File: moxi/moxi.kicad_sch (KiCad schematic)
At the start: 7 parts, among them M3 Motor_Servo, M4 Motor_Servo, SW1 SW_SPST, U1 MAX98357A, U2 ProMicro_2

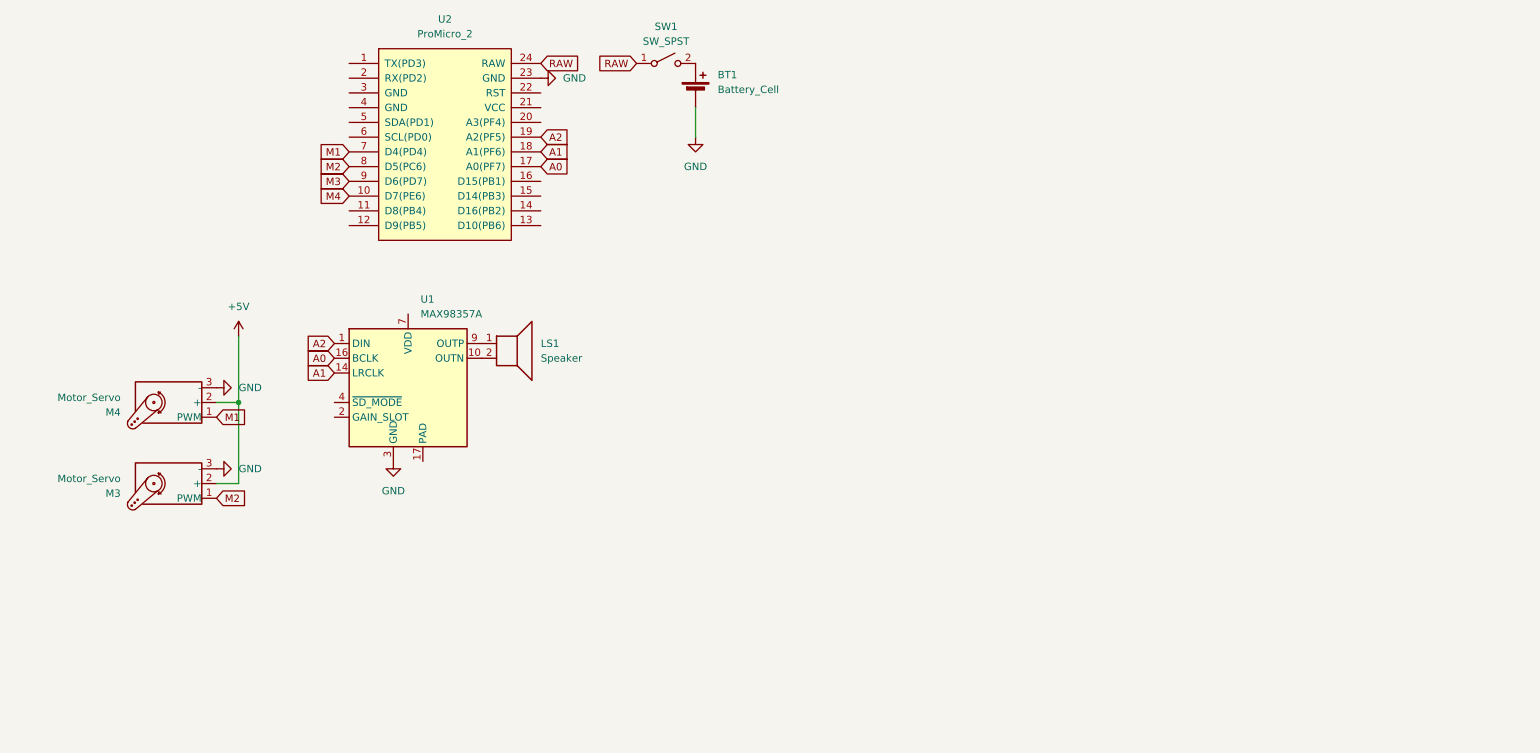
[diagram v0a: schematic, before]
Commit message: Update schematic
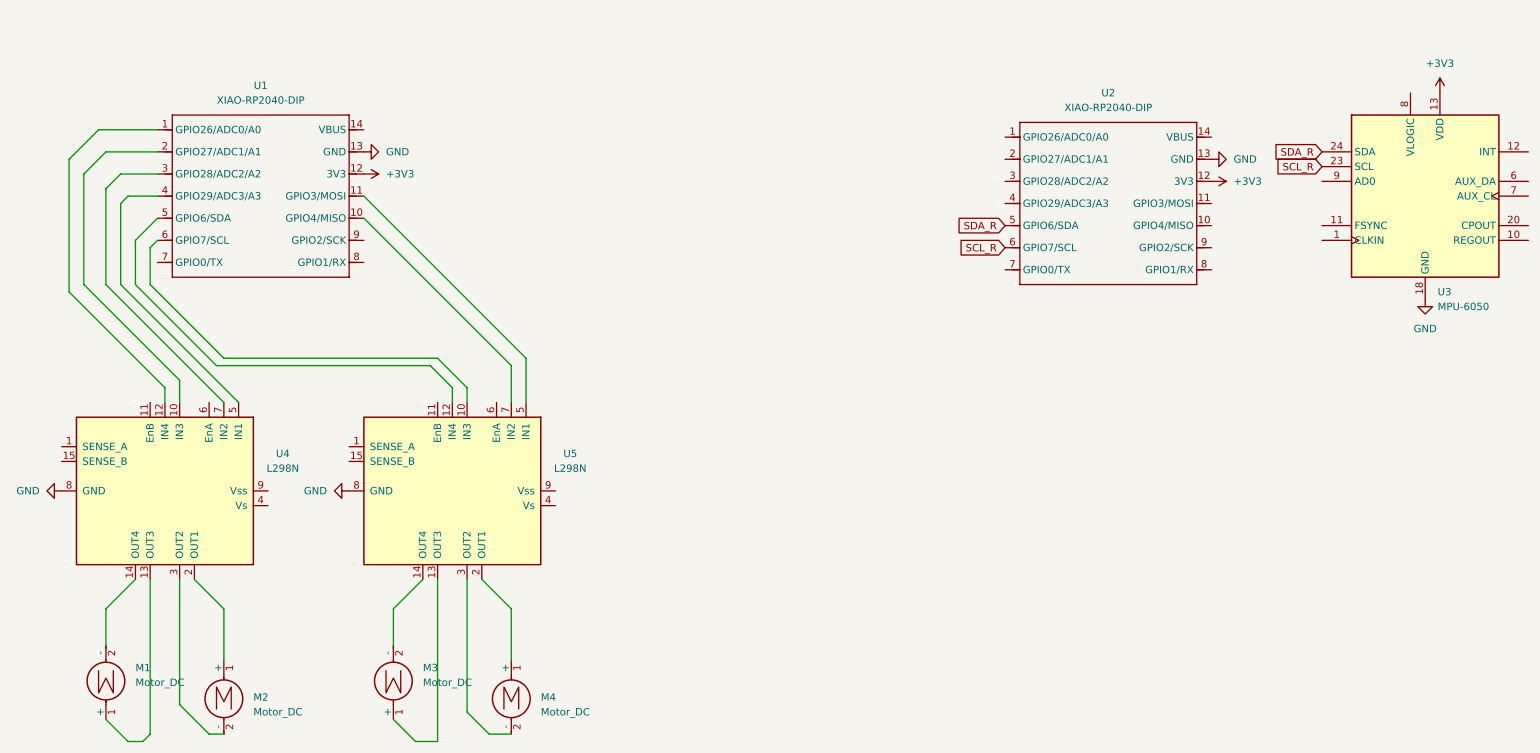
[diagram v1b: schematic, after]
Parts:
- removed BT1: Battery_Cell, Connector_JST:JST_PH_S2B-PH-K_1x02_P2.00mm_Horizontal, symbol Device:Battery_Cell
- removed LS1: Speaker, symbol Device:Speaker
- removed M3, M4: Motor_Servo, symbol Motor:Motor_Servo
- removed SW1: SW_SPST, Button_Switch_THT:SW_SPST_Omron_B3F-40xx, symbol Switch:SW_SPST
- removed U1: MAX98357A, Package_DFN_QFN:TQFN-16-1EP_3x3mm_P0.5mm_EP1.23x1.23mm, symbol Audio:MAX98357A
- removed U2: ProMicro_2, symbol nRF52840:ProMicro_2
- added M1, M2, M3, M4: Motor_DC, symbol Motor:Motor_DC
- added U1, U2: XIAO-RP2040-DIP, Module:MOUDLE14P-XIAO-DIP-SMD, symbol xiao:XIAO-RP2040-DIP
- added U3: MPU-6050, Sensor_Motion:InvenSense_QFN-24_4x4mm_P0.5mm, symbol Sensor_Motion:MPU-6050
- added U4, U5: L298N, Package_TO_SOT_THT:TO-220-15_P2.54x2.54mm_StaggerOdd_Lead4.58mm_Vertical, symbol Driver_Motor:L298N
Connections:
- net GND: now also U1.13 (GND), U2.13 (GND), U3.18 (GND), U4.8 (GND), U5.8 (GND)
- new net: M1.1 (+), U4.13 (OUT3)
- new net: M1.2 (-), U4.14 (OUT4)
- new net: M4.1 (+), U5.2 (OUT1)
- new net: M4.2 (-), U5.3 (OUT2)
- new net: U1.2 (GPIO27/ADC1/A1), U4.10 (IN3)
- new net: U1.1 (GPIO26/ADC0/A0), U4.12 (IN4)
- new net: M2.1 (+), U4.2 (OUT1)
- new net: M2.2 (-), U4.3 (OUT2)
- new net: U1.4 (GPIO29/ADC3/A3), U4.5 (IN1)
- new net: U1.3 (GPIO28/ADC2/A2), U4.7 (IN2)
- new net: U1.10 (GPIO4/MISO), U5.7 (IN2)
- new net: U1.11 (GPIO3/MOSI), U5.5 (IN1)
- new net: U1.5 (GPIO6/SDA), U5.12 (IN4)
- new net: U1.6 (GPIO7/SCL), U5.10 (IN3)
- new net: M3.1 (+), U5.13 (OUT3)
- new net: M3.2 (-), U5.14 (OUT4)
- new net +3V3: U1.12 (3V3), U2.12 (3V3), U3.13 (VDD)
- new net SCL_R: U2.6 (GPIO7/SCL), U3.23 (SCL)
- new net SDA_R: U2.5 (GPIO6/SDA), U3.24 (SDA)
